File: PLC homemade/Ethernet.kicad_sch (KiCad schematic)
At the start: 35 parts, among them U3 W5500, Y1 Crystal

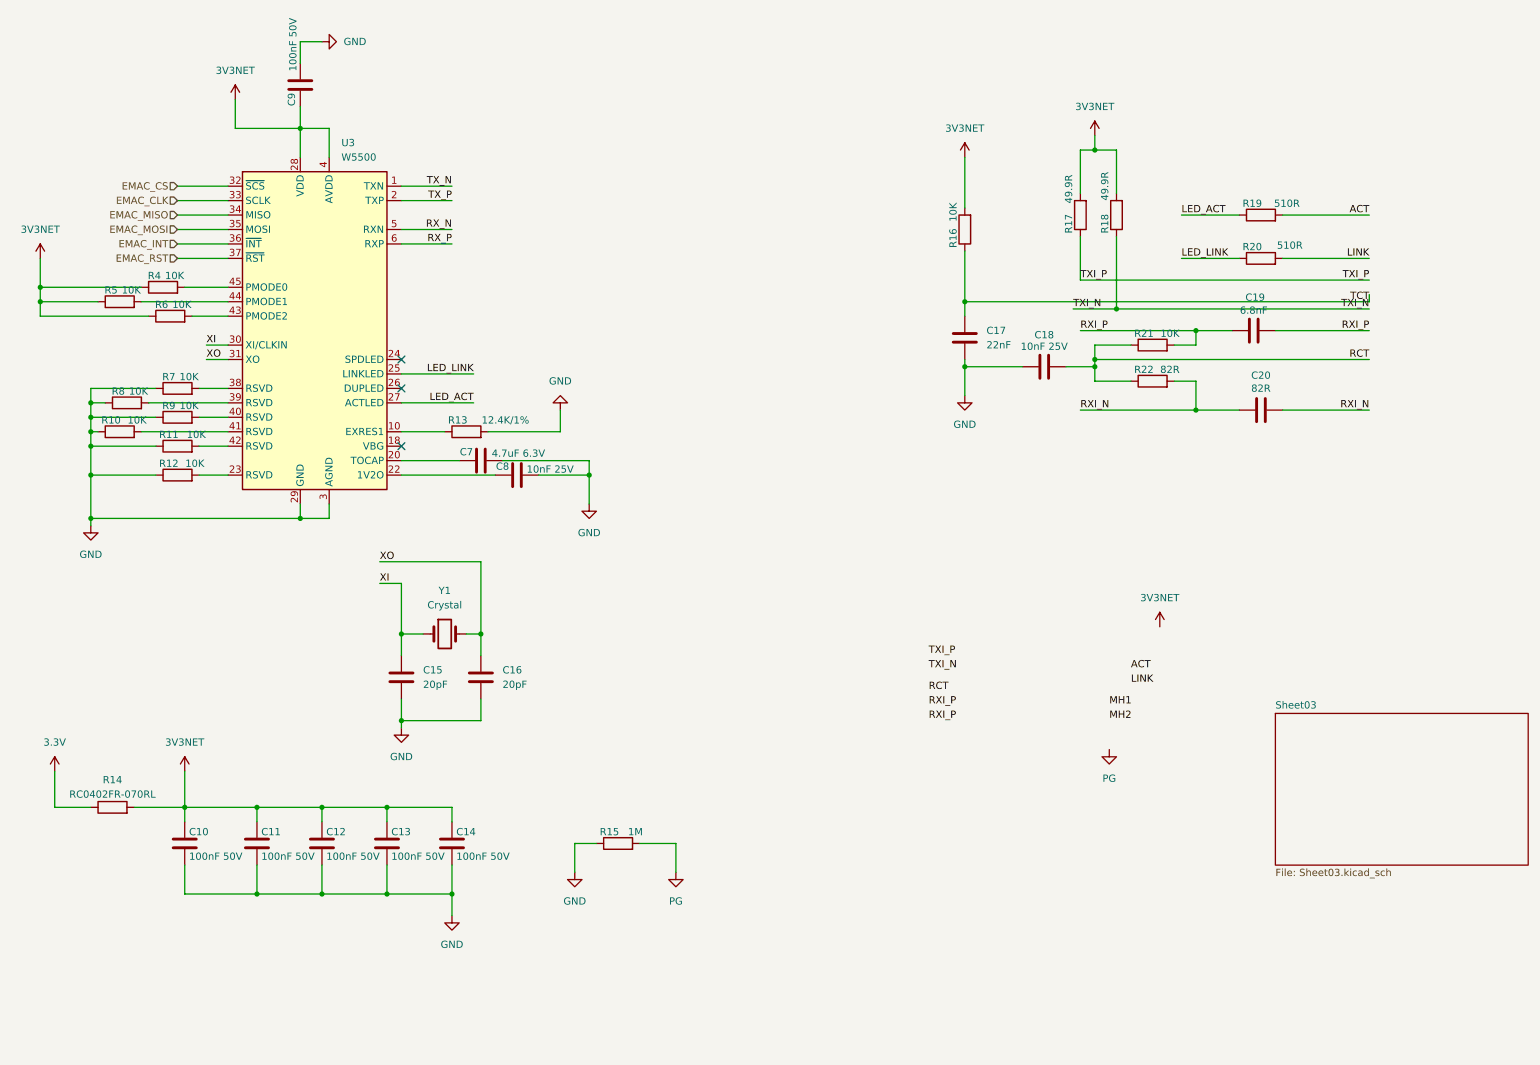
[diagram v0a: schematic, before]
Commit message: :art: COMPLETED SHEET3
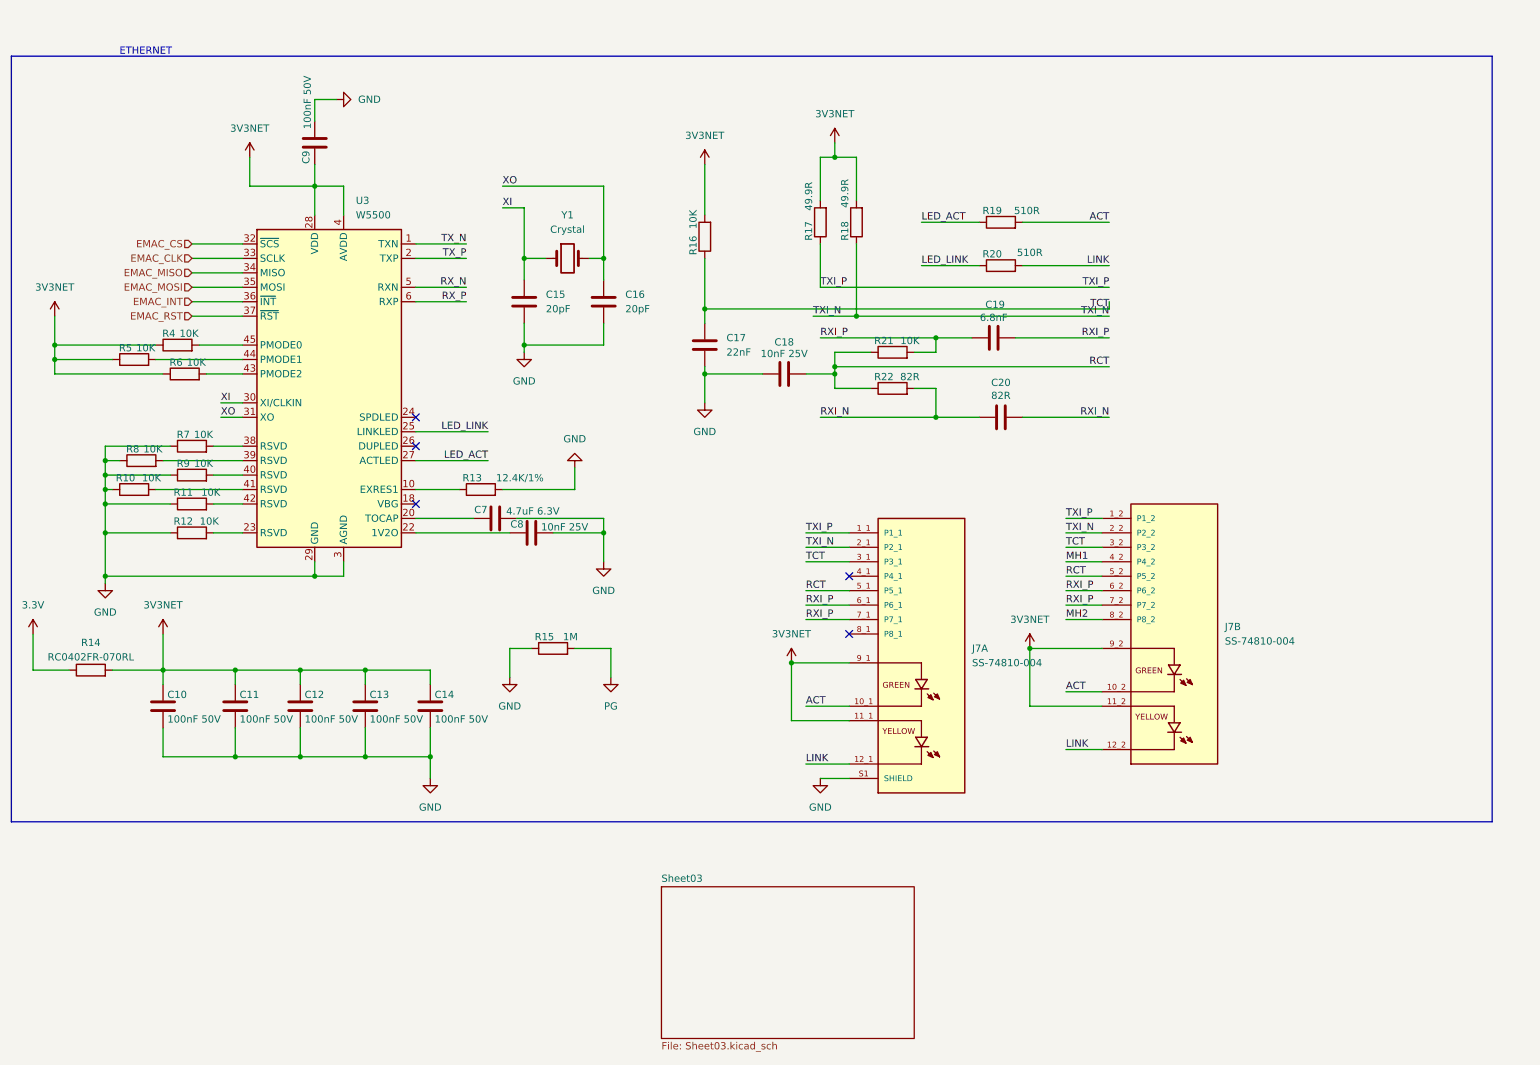
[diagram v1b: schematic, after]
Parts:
- added J7: SS-74810-004, SS-74810-004:BEL_SS-74810-004, symbol SS-74810-004:SS-74810-004
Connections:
- net 3V3NET: now also J7.11_1, J7.11_2, J7.9_1, J7.9_2
- net ACT: now also J7.10_1, J7.10_2
- net GND: now also J7.S1 (SHIELD), J7.S2 (SHIELD), J7.S3 (SHIELD), J7.S4 (SHIELD), J7.S5 (SHIELD), J7.S6 (SHIELD), J7.S7 (SHIELD), J7.S8 (SHIELD), J7.S9 (SHIELD)
- net LINK: now also J7.12_1, J7.12_2
- net MH1: now also J7.4_2 (P4_2)
- net MH2: now also J7.8_2 (P8_2)
- net RCT: now also J7.5_1 (P5_1), J7.5_2 (P5_2)
- net RXI_P: now also J7.6_1 (P6_1), J7.6_2 (P6_2), J7.7_1 (P7_1), J7.7_2 (P7_2)
- net TCT: now also J7.3_1 (P3_1), J7.3_2 (P3_2)
- net TXI_N: now also J7.2_1 (P2_1), J7.2_2 (P2_2)
- net TXI_P: now also J7.1_1 (P1_1), J7.1_2 (P1_2)
- no-connect marks 3 -> 5
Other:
- note added: "ETHERNET"
- moved on the sheet: C10, C11, C12, C13, C14, C15, C16, C17, C18, C19, C20, C7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

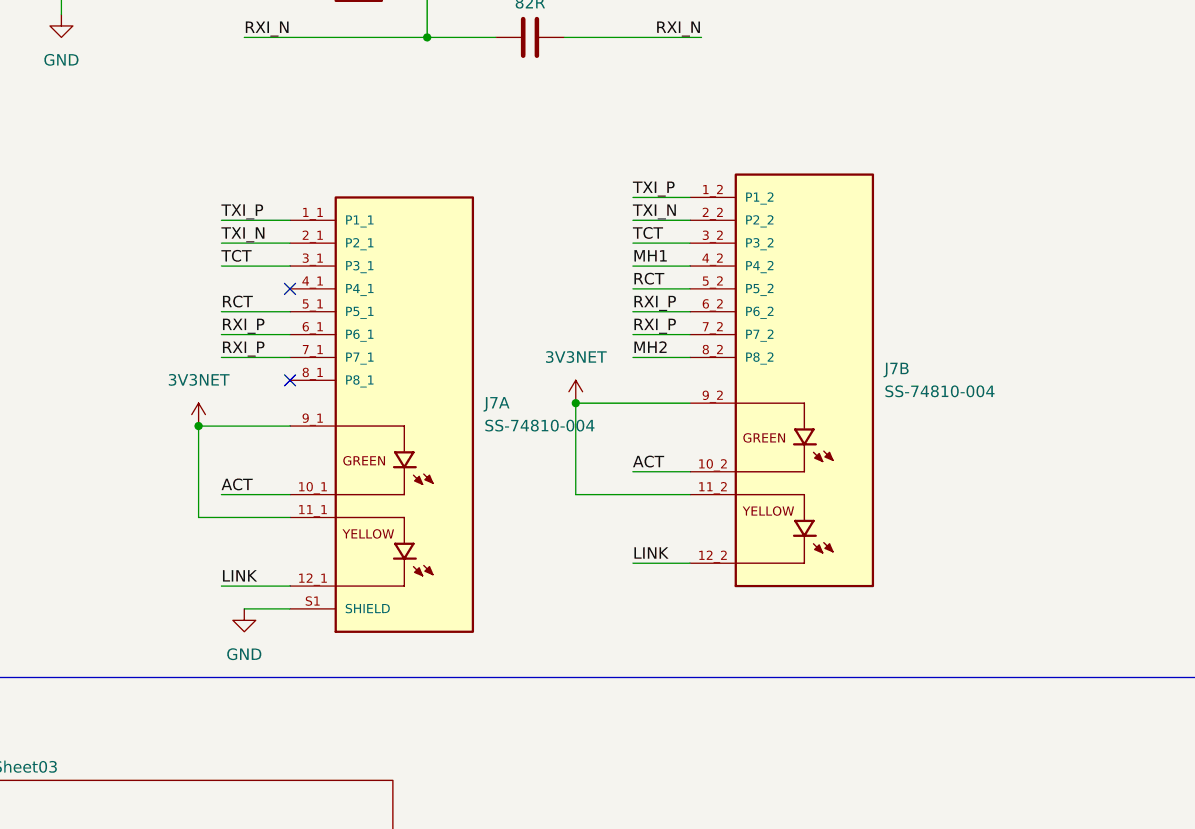
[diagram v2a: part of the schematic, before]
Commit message: :clown_face: changed HEIRACHIAL to global
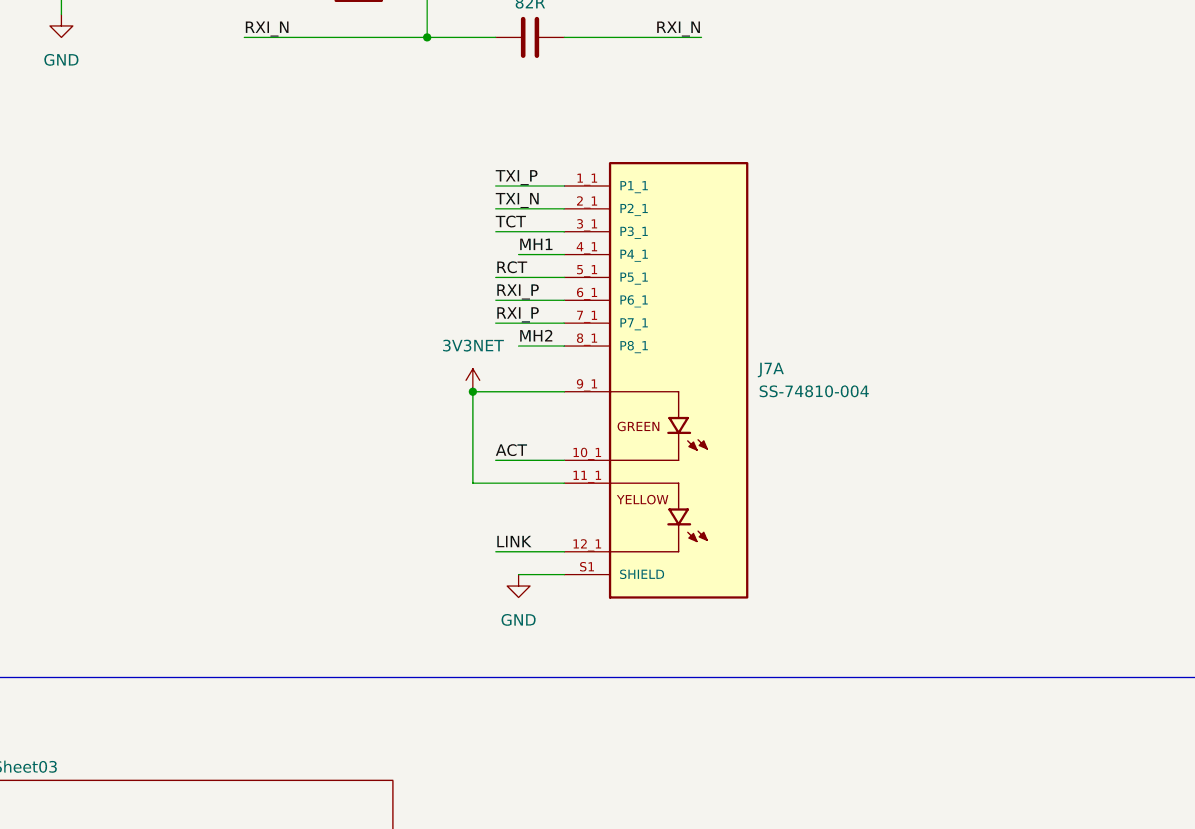
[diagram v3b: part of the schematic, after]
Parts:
- removed unit 2 of J7
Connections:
- net MH1: now also J7.4_1 (P4_1)
- net MH2: now also J7.8_1 (P8_1)
- no-connect marks 5 -> 3
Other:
- moved on the sheet: J7A

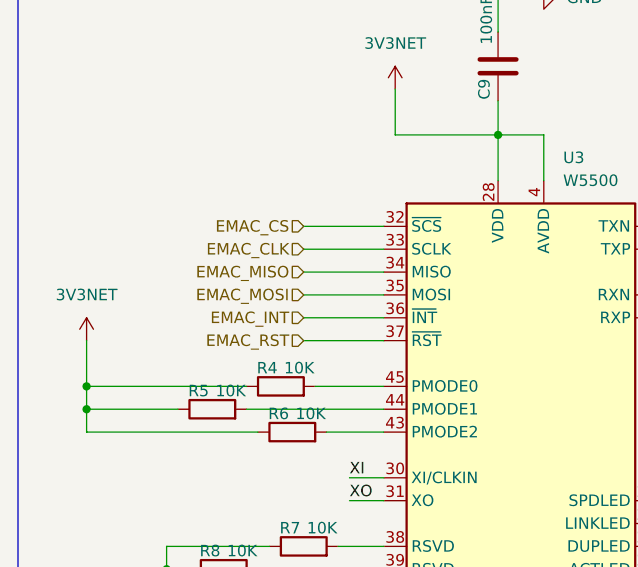
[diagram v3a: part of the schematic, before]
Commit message: :tada: Added small changes
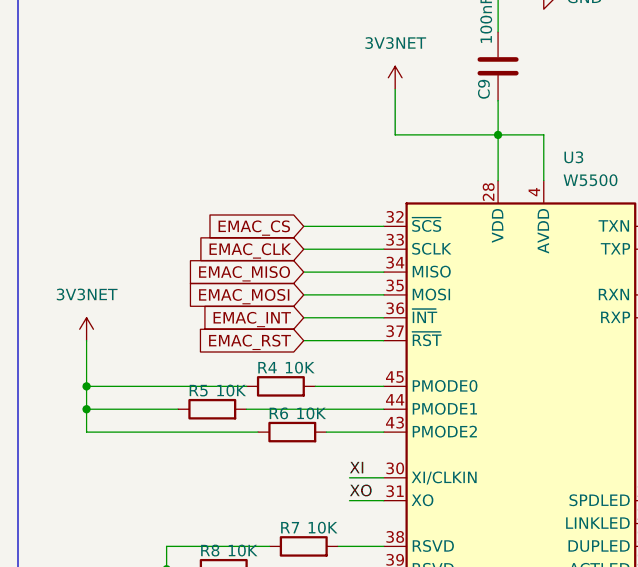
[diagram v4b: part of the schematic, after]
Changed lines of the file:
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@@
 		)
 	)
-	(hierarchical_label "EMAC_INT"
+	(global_label "EMAC_RST"
 		(shape input)
-		(at 46.99 64.77 180)
+		(at 46.99 67.31 180)
+		(fields_autoplaced yes)
 		(effects
 			(font
@@
 			(justify right)
 		)
+		(property "Intersheetrefs" "${INTERSHEET_REFS}"
+			(at 34.6311 67.31 0)
+			(effects
+				(font
+					(size 1.27 1.27)
+				)
+				(justify right)
+				(hide yes)
+			)
+		)
 	)
-	(hierarchical_label "EMAC_MOSI"
+	(global_label "EMAC_INT"
 		(shape input)
-		(at 46.99 62.23 180)
+		(at 46.99 64.77 180)
+		(fields_autoplaced yes)
 		(effects
 			(font
@@
 			(justify right)
 		)
+		(property "Intersheetrefs" "${INTERSHEET_REFS}"
+			(at 35.1753 64.77 0)
+			(effects
+				(font
+					(size 1.27 1.27)
+				)
+				(justify right)
+				(hide yes)
+			)
+		)
 	)
-	(hierarchical_label "EMAC_MISO"
+	(global_label "EMAC_MOSI"
 		(shape input)
-		(at 46.99 59.69 180)
+		(at 46.99 62.23 180)
+		(fields_autoplaced yes)
 		(effects
 			(font
@@
 			(justify right)
 		)
+		(property "Intersheetrefs" "${INTERSHEET_REFS}"
+			(at 33.482 62.23 0)
+			(effects
+				(font
+					(size 1.27 1.27)
+				)
+				(justify right)
+				(hide yes)
+			)
+		)
 	)
-	(hierarchical_label "EMAC_CLK"
+	(global_label "EMAC_MISO"
 		(shape input)
-		(at 46.99 57.15 180)
+		(at 46.99 59.69 180)
+		(fields_autoplaced yes)
 		(effects
 			(font
@@
 			(justify right)
 		)
+		(property "Intersheetrefs" "${INTERSHEET_REFS}"
+			(at 33.482 59.69 0)
+			(effects
+				(font
+					(size 1.27 1.27)
+				)
+				(justify right)
+				(hide yes)
+			)
+		)
 	)
-	(hierarchical_label "EMAC_CS"
+	(global_label "EMAC_CLK"
 		(shape input)
-		(at 46.99 54.61 180)
+		(at 46.99 57.15 180)
+		(fields_autoplaced yes)
 		(effects
 			(font
@@
 			(justify right)
 		)
+		(property "Intersheetrefs" "${INTERSHEET_REFS}"
+			(at 34.5101 57.15 0)
+			(effects
+				(font
+					(size 1.27 1.27)
+				)
+				(justify right)
+				(hide yes)
+			)
+		)
 	)
-	(hierarchical_label "EMAC_RST"
+	(global_label "EMAC_CS"
 		(shape input)
-		(at 46.99 67.31 180)
+		(at 46.99 54.61 180)
+		(fields_autoplaced yes)
 		(effects
 			(font
@@
 			(justify right)
 		)
+		(property "Intersheetrefs" "${INTERSHEET_REFS}"
+			(at 35.5987 54.61 0)
+			(effects
+				(font
+					(size 1.27 1.27)
+				)
+				(justify right)
+				(hide yes)
+			)
+		)
 	)
